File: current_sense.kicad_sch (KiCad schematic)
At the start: 1 part, among them IC4 AD8030ARZ

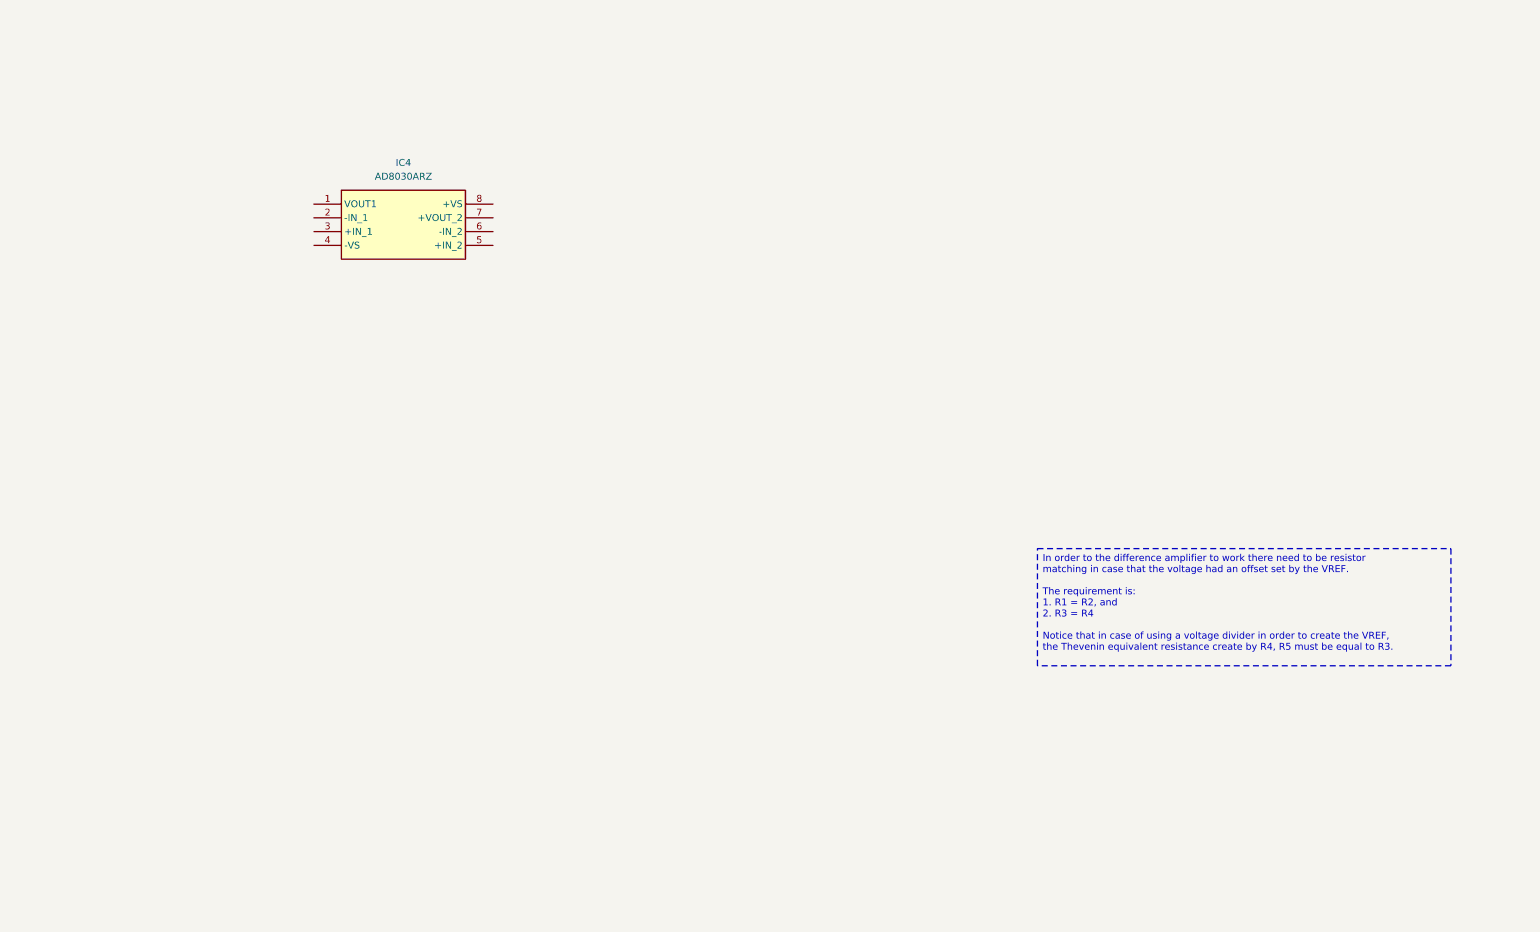
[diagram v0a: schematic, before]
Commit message: Initial layout
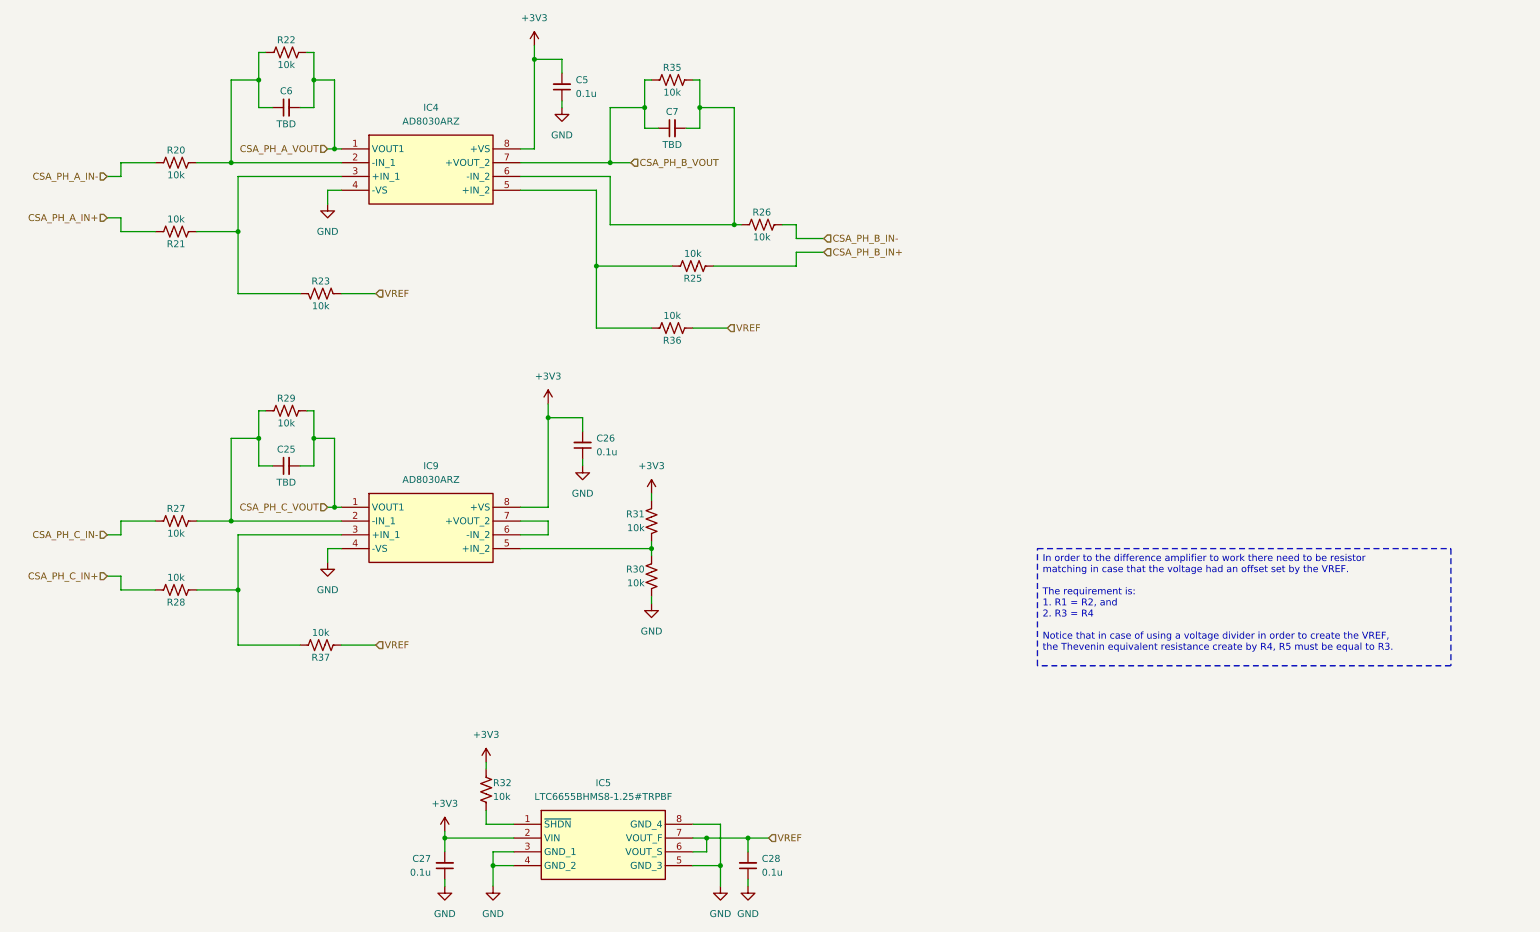
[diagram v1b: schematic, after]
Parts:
- added C25, C6, C7: TBD, Capacitor_SMD:C_0603_1608Metric, symbol Device:C_Small
- added C26, C27, C28, C5: 0.1u, Capacitor_SMD:C_0603_1608Metric, symbol Device:C_Small
- added IC5: LTC6655BHMS8-1.25#TRPBF, BLDC-Motor-Driver:LTC6655, symbol BLDC-Motor-Driver_v2:LTC6655BHMS8-1.25#TRPBF
- added IC9: AD8030ARZ, BLDC-Motor-Driver:AD8030ARZ-SOIC8, symbol bldc-driver-pcb:AD8030ARZ
- added R20, R21, R22, R23, R25, R26, R27, R28, R29, R30, R31, R32, R35, R36, R37: 10k, Resistor_SMD:R_0603_1608Metric, symbol Device:R_US
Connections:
- net CSA_PH_A_VOUT: now reaches IC4.1 (VOUT1)
- net CSA_PH_A_VOUT: now also C6.2, R22.2
- net at IC4.2 (-IN_1): now also C6.1, R20.2, R22.1
- net at IC4.3 (+IN_1): now also R21.1, R23.2
- net GND: now reaches IC4.4 (-VS)
- net GND: now also C26.1, C27.1, C28.1, C5.1, IC5.3 (GND_1), IC5.4 (GND_2), IC5.5 (GND_3), IC5.8 (GND_4), IC9.4 (-VS), R30.2
- net at IC4.5 (+IN_2): now also R25.2, R36.2
- net at IC4.6 (-IN_2): now also C7.2, R26.1, R35.2
- net CSA_PH_B_VOUT: now reaches IC4.7 (+VOUT_2)
- net CSA_PH_B_VOUT: now also C7.1, R35.1
- net +3V3: now reaches IC4.8 (+VS)
- net +3V3: now also C26.2, C27.2, C5.2, IC5.2 (VIN), IC9.8 (+VS), R31.1, R32.1
- new net: IC9.3 (+IN_1), R28.1, R37.2
- new net: C25.1, IC9.2 (-IN_1), R27.2, R29.1
- new net: IC5.1 (~{SHDN}), R32.2
- new net: IC9.5 (+IN_2), R30.1, R31.2
- new net: IC9.6 (-IN_2), IC9.7 (+VOUT_2)
- new net CSA_PH_A_IN+: R21.2
- new net CSA_PH_A_IN-: R20.1
- new net CSA_PH_B_IN+: R25.1
- new net CSA_PH_B_IN-: R26.2
- new net CSA_PH_C_IN+: R28.2
- new net CSA_PH_C_IN-: R27.1
- new net CSA_PH_C_VOUT: C25.2, IC9.1 (VOUT1), R29.2
- new net VREF: C28.2, IC5.6 (VOUT_S), IC5.7 (VOUT_F), R23.1, R36.1, R37.1
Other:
- moved on the sheet: IC4
